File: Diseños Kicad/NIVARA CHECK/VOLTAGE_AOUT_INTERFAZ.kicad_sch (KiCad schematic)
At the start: 4 parts, among them U6 XTR116U

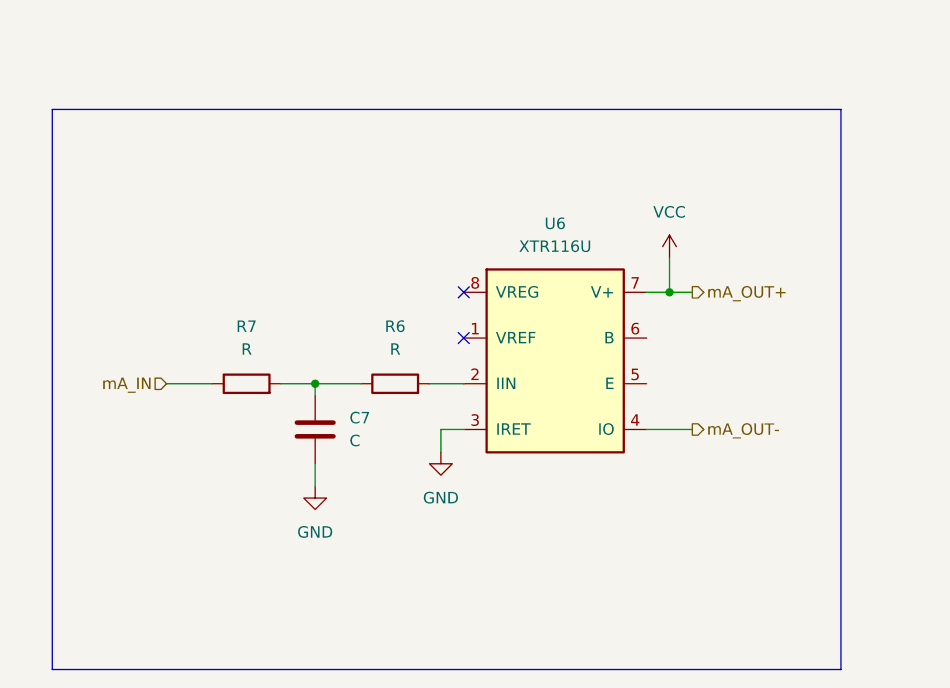
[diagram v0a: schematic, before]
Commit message: ACTUALIZACION HECHA
PCB SUPUESTA
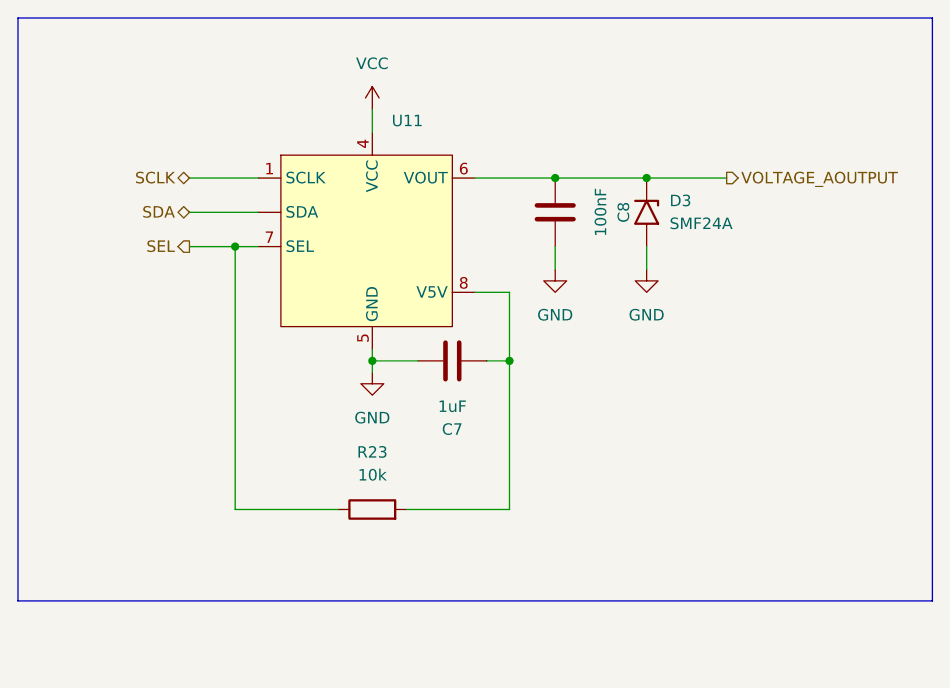
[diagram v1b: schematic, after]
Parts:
- removed R6, R7: R, symbol Device:R
- removed U6: XTR116U, Package_SO:SOIC-8_3.9x4.9mm_P1.27mm, symbol Interface_CurrentLoop:XTR116U
- added C8: 100nF, symbol Device:C
- added D3: SMF24A, Diode_SMD:D_SMF, symbol Diode:SMF24A
- added R23: 10k, symbol Device:R
- added U11: ~, Riqi_Parts:eSOP-8, symbol Riqi_Parts:GP8201S
- C7: value C -> 1uF
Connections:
- net GND: now also C7.1, C8.1, D3.2 (A2), U11.5 (GND); no longer C7.2
- net VCC: now also U11.4 (VCC)
- new net: C7.2, R23.2, U11.8 (V5V)
- new net SCLK: U11.1 (SCLK)
- new net SDA: U11. (SDA)
- new net SEL: R23.1, U11.7 (SEL)
- new net VOLTAGE_AOUTPUT: C8.2, D3.1 (A1), U11.6 (VOUT)
- no-connect marks 2 -> 0
